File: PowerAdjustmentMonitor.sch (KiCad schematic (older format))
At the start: 35 parts, among them U5 LM337T, U6 LM337T, U7 LM317T, U8 LM317T

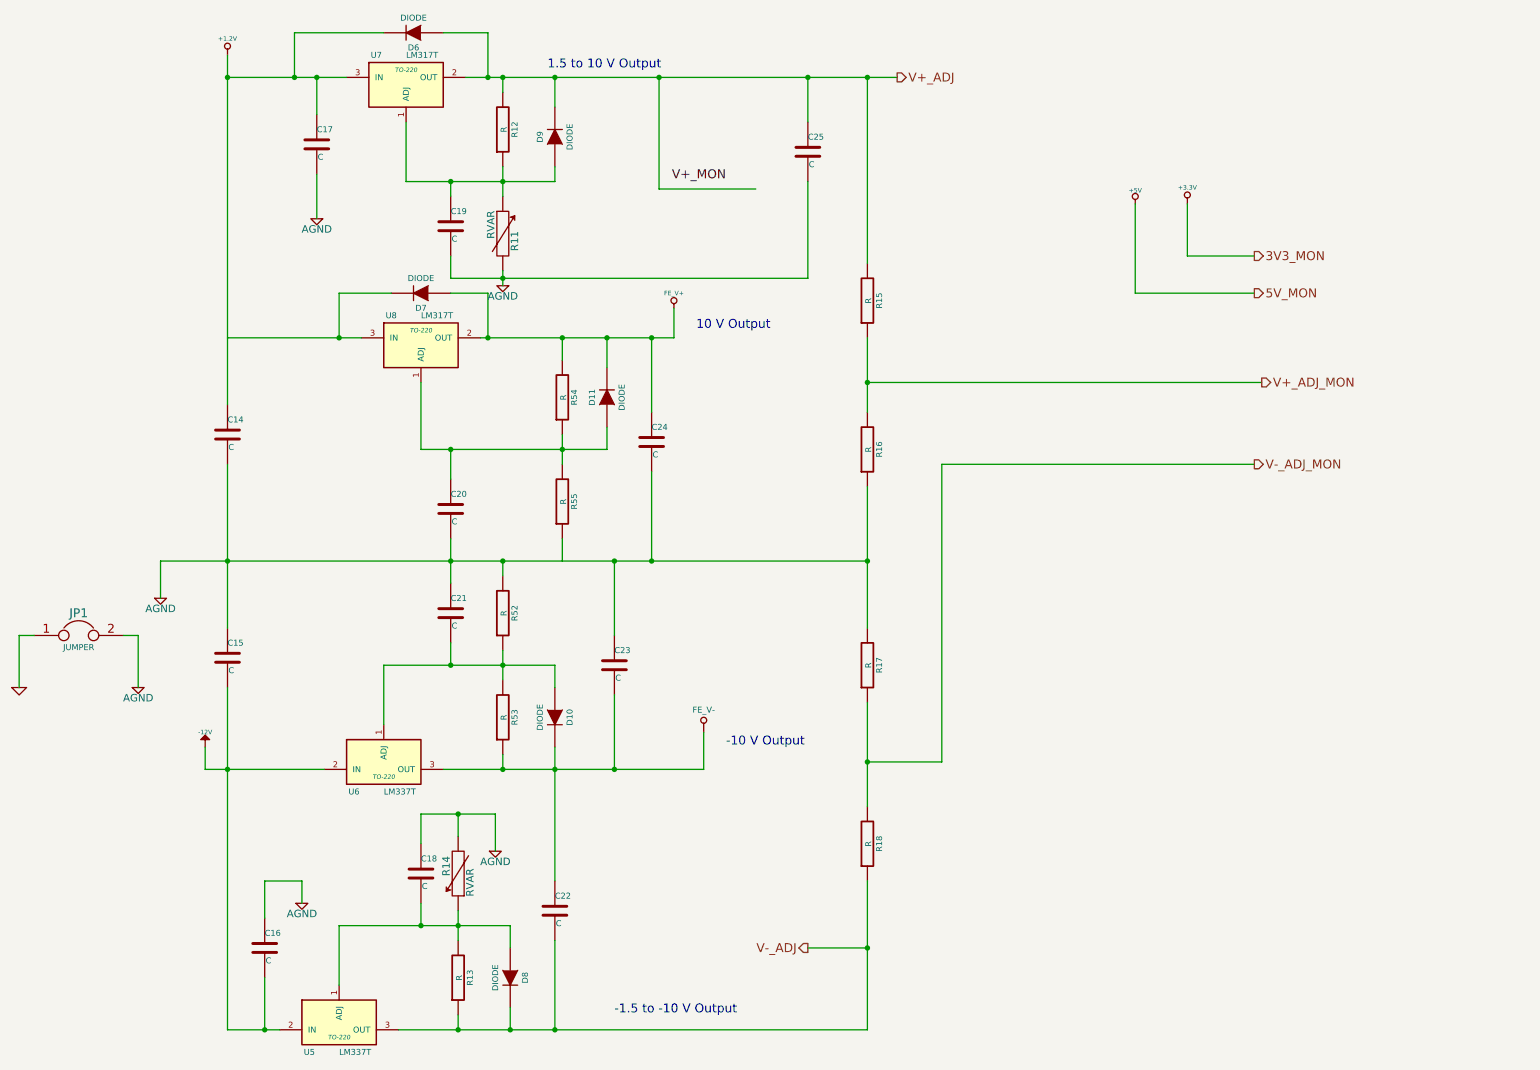
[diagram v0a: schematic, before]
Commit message: Layout sessions 1-4.
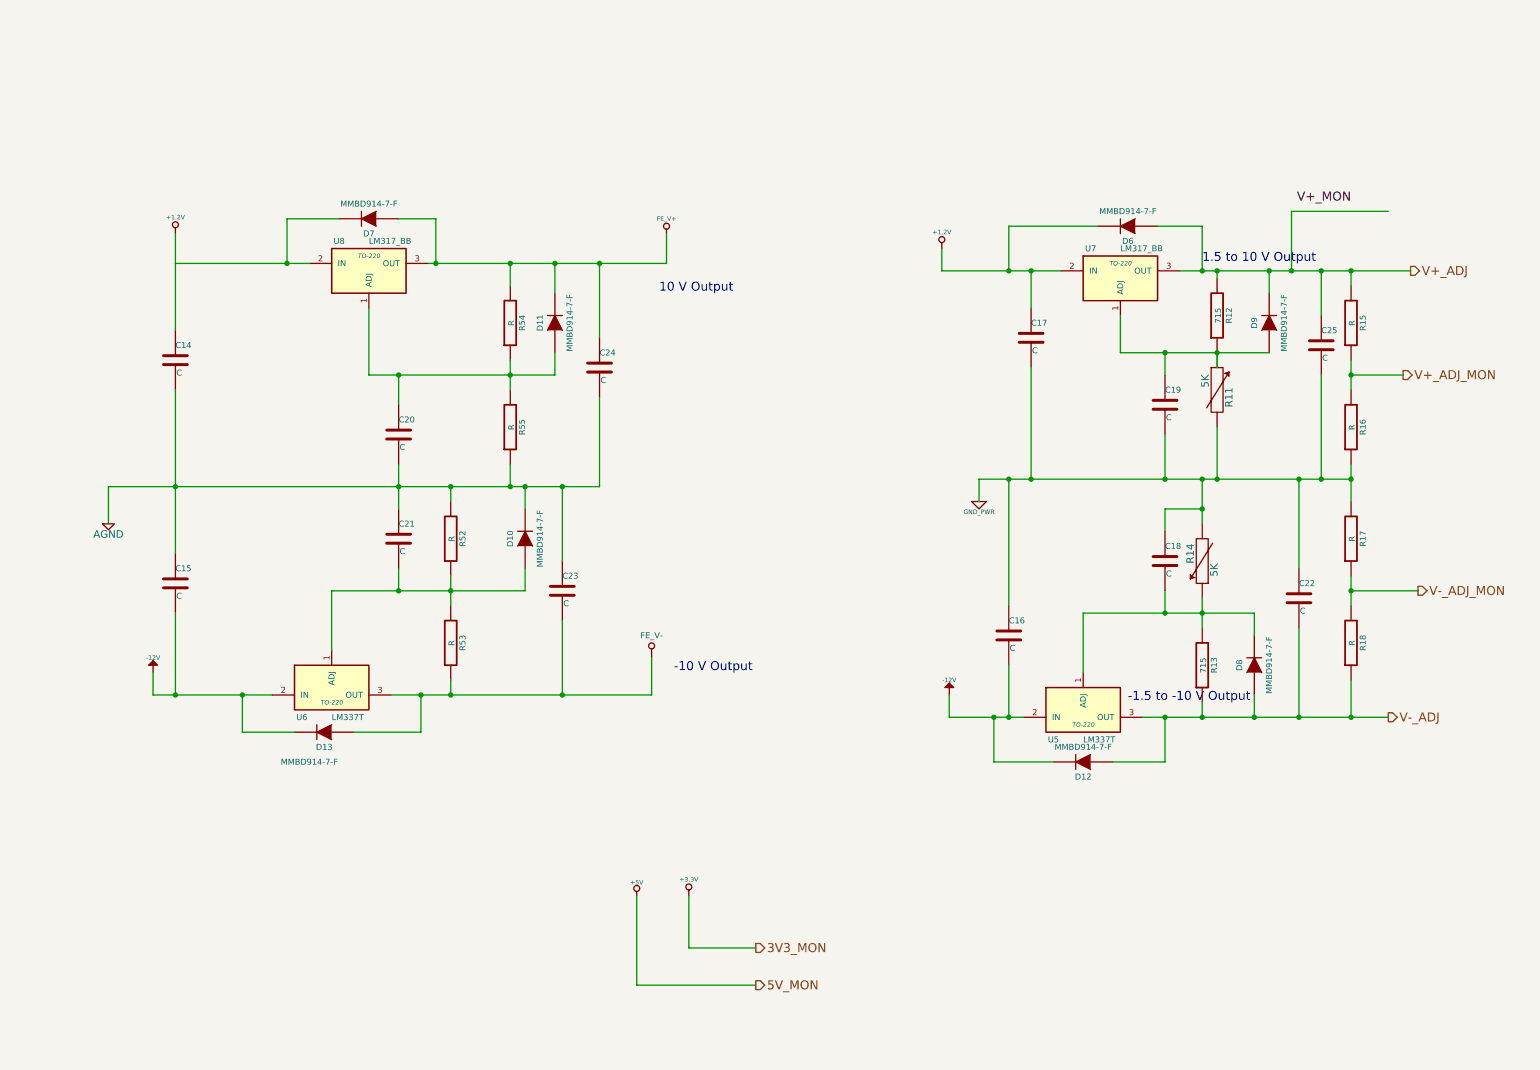
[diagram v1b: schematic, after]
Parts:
- removed JP1: JUMPER, symbol JUMPER
- removed U7, U8: LM317T, TO-220, symbol LM317T
- added D12, D13: MMBD914-7-F, symbol DIODE
- added U7, U8: LM317_BB, TO-220, symbol LM317_BB
- D10, D11, D6, D7, D8: value DIODE -> MMBD914-7-F; MFG Part Number (none) -> MMBD914-7-F; MFG name (none) -> Diodes Inc
- D9: value DIODE -> MMBD914-7-F; MFG Part Number (none) -> MMBD914-7-F; MFG name (none) -> DiodeS Inc
- R11, R14: value RVAR -> 5K
- R12, R13: value R -> 715
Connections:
- net +1.2V: now also U7.2 (IN)
- net -12V: now also D12.2 (K), D13.2 (K)
- net AGND: now also D10.2 (K), R55.1; no longer C16.1, C17.2, C18.1, C19.2, C25.2, R11.2, R14.2, R16.1, R17.2
- net FE_V+: now also U8.3 (OUT)
- net FE_V-: now also D13.1 (A); no longer C22.1, D10.2 (K)
- net V+_ADJ: now also U7.3 (OUT)
- net V-_ADJ: now also D8.1 (A), D12.1 (A); no longer D8.2 (K)
- net at C19.1, D9.1 (A), R11.1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: now also U7.1 (ADJ)
- net at C20.1, D11.1 (A), R54.1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: now also U8.1 (ADJ)
- net at D7.2 (K): now also U8.2 (IN)
- net at C18.2, R13.2, R14.1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: now also D8.2 (K); no longer D8.1 (A)
- new net GND_PWR: C16.1, C17.2, C18.1, C19.2, C22.1, C25.2, R11.2, R14.2, R16.1, R17.2
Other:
- moved on the sheet: C14, C15, C16, C17, C18, C19, C20, C21, C22, C23, C24, C25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
